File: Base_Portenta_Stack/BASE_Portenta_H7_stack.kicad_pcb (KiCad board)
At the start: 2 copper layers, 79.8 x 26.6 mm, 8 parts, among them J4 PinHeader_1x04_P2.00mm_Vertic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

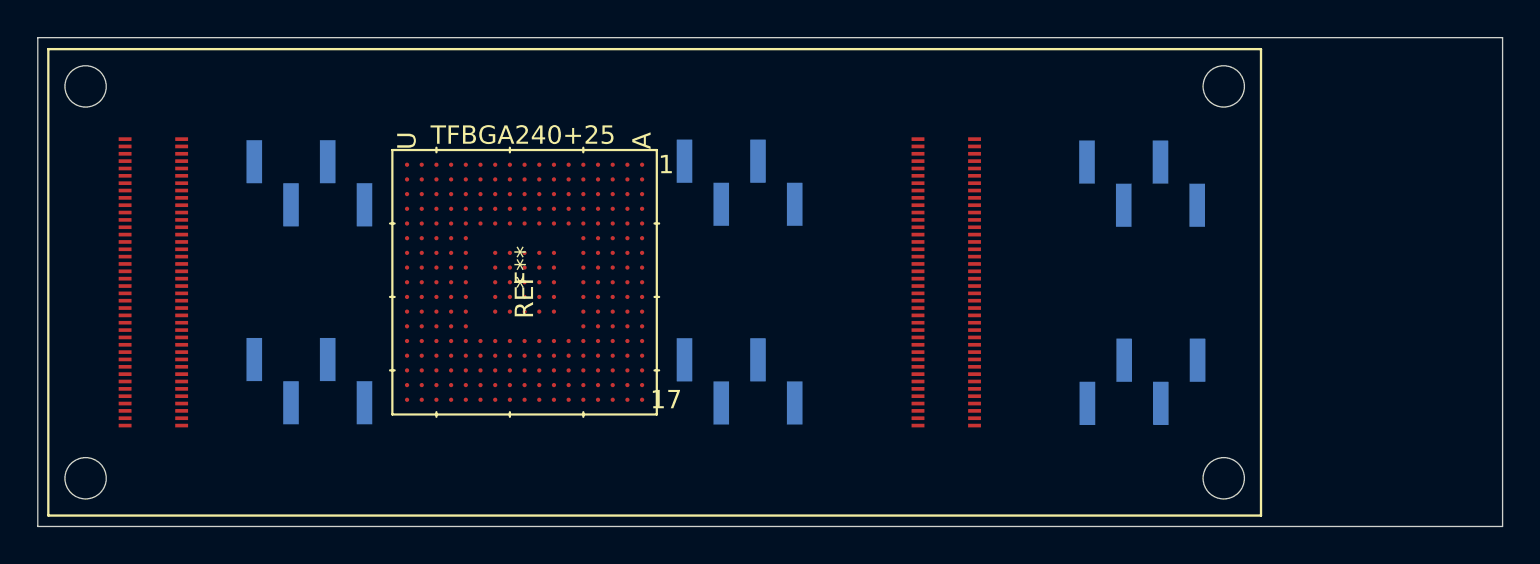
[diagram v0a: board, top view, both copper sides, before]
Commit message: Updade
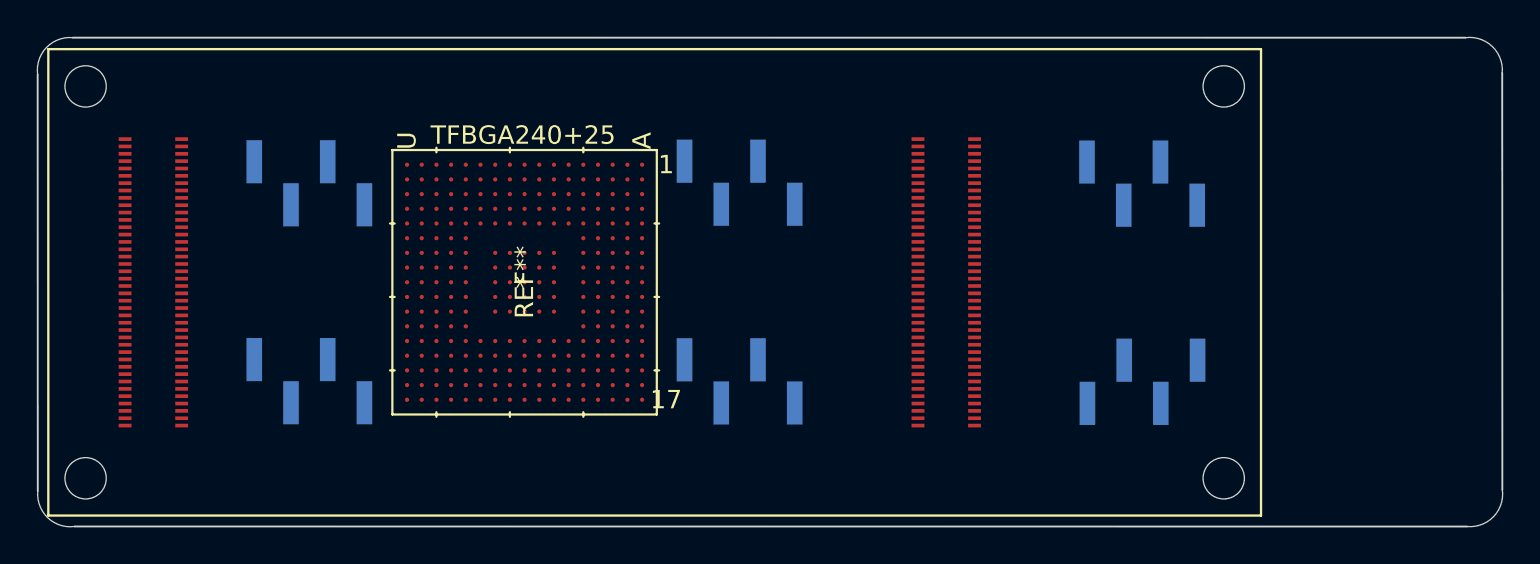
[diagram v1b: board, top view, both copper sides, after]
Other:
- outline, holes or cut-outs redrawn
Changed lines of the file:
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@@
       )
     )
-    (model "${KIPRJMOD}/Arduino-Portenta-H7-STEP-A210428.step"
+    (model "C:/Users/45262/Documents/GitHub/MTBeDRIVE/img/DF40C(2.0)-80DS.stp"
+      (offset (xyz 0.1 15.9 0.5))
+      (scale (xyz 1 1 1))
+      (rotate (xyz 90 -180 90))
+    )
+    (model "C:/Users/45262/Documents/GitHub/MTBeDRIVE/img/DF40C(2.0)-80DS.stp"
+      (offset (xyz -0.1 -27.3 0.5))
+      (scale (xyz 1 1 1))
+      (rotate (xyz -90 0 90))
+    )
+    (model "C:/Users/45262/Desktop/NRF_HALLA/Arduino-Portenta-H7-STEP-A210428.step"
       (offset (xyz 0 0 2))
       (scale (xyz 1 1 1))
@@
     )
   )
-  (gr_rect (start 106.21 80.47) (end 185.98 107.09) (layer "Edge.Cuts") (width 0.05) (fill none))
+  (gr_arc (start 183.950563 80.472791) (mid 185.42 80.95) (end 185.960563 82.392791) (layer "Edge.Cuts") (width 0.05))
+  (gr_line (start 184.047772 107.093354) (end 108.22 107.09) (layer "Edge.Cuts") (width 0.1))
+  (gr_arc (start 185.967772 105.083354) (mid 185.490563 106.552791) (end 184.047772 107.093354) (layer "Edge.Cuts") (width 0.05))
+  (gr_arc (start 108.22 107.09) (mid 106.750563 106.612791) (end 106.21 105.17) (layer "Edge.Cuts") (width 0.05))
+  (gr_line (start 108.122791 80.469437) (end 183.950563 80.472791) (layer "Edge.Cuts") (width 0.1))
+  (gr_arc (start 106.202791 82.479437) (mid 106.68 81.01) (end 108.122791 80.469437) (layer "Edge.Cuts") (width 0.05))
+  (gr_line (start 106.21 105.17) (end 106.202791 82.479437) (layer "Edge.Cuts") (width 0.1))
+  (gr_line (start 185.960563 82.392791) (end 185.967772 105.083354) (layer "Edge.Cuts") (width 0.1))
 )
